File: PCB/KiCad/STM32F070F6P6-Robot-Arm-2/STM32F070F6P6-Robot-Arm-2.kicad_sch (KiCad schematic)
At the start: 37 parts, among them J10 Barrel_Jack_Switch, J6 Conn_01x03_Pin, J7 Conn_01x03_Pin, J8 Conn_01x03_Pin, J9 Conn_01x03_Pin, T14C1_LED1 LED, T1C2_LED1 LED, T1C3_LED1 LED, T3C1_LED1 LED, T3C2_LED1 LED, T3C4_LED1 LED, U1 STM32F070F6Px, U2_AMS1117-3.3 AMS1117-3.3, Y1 8MHz

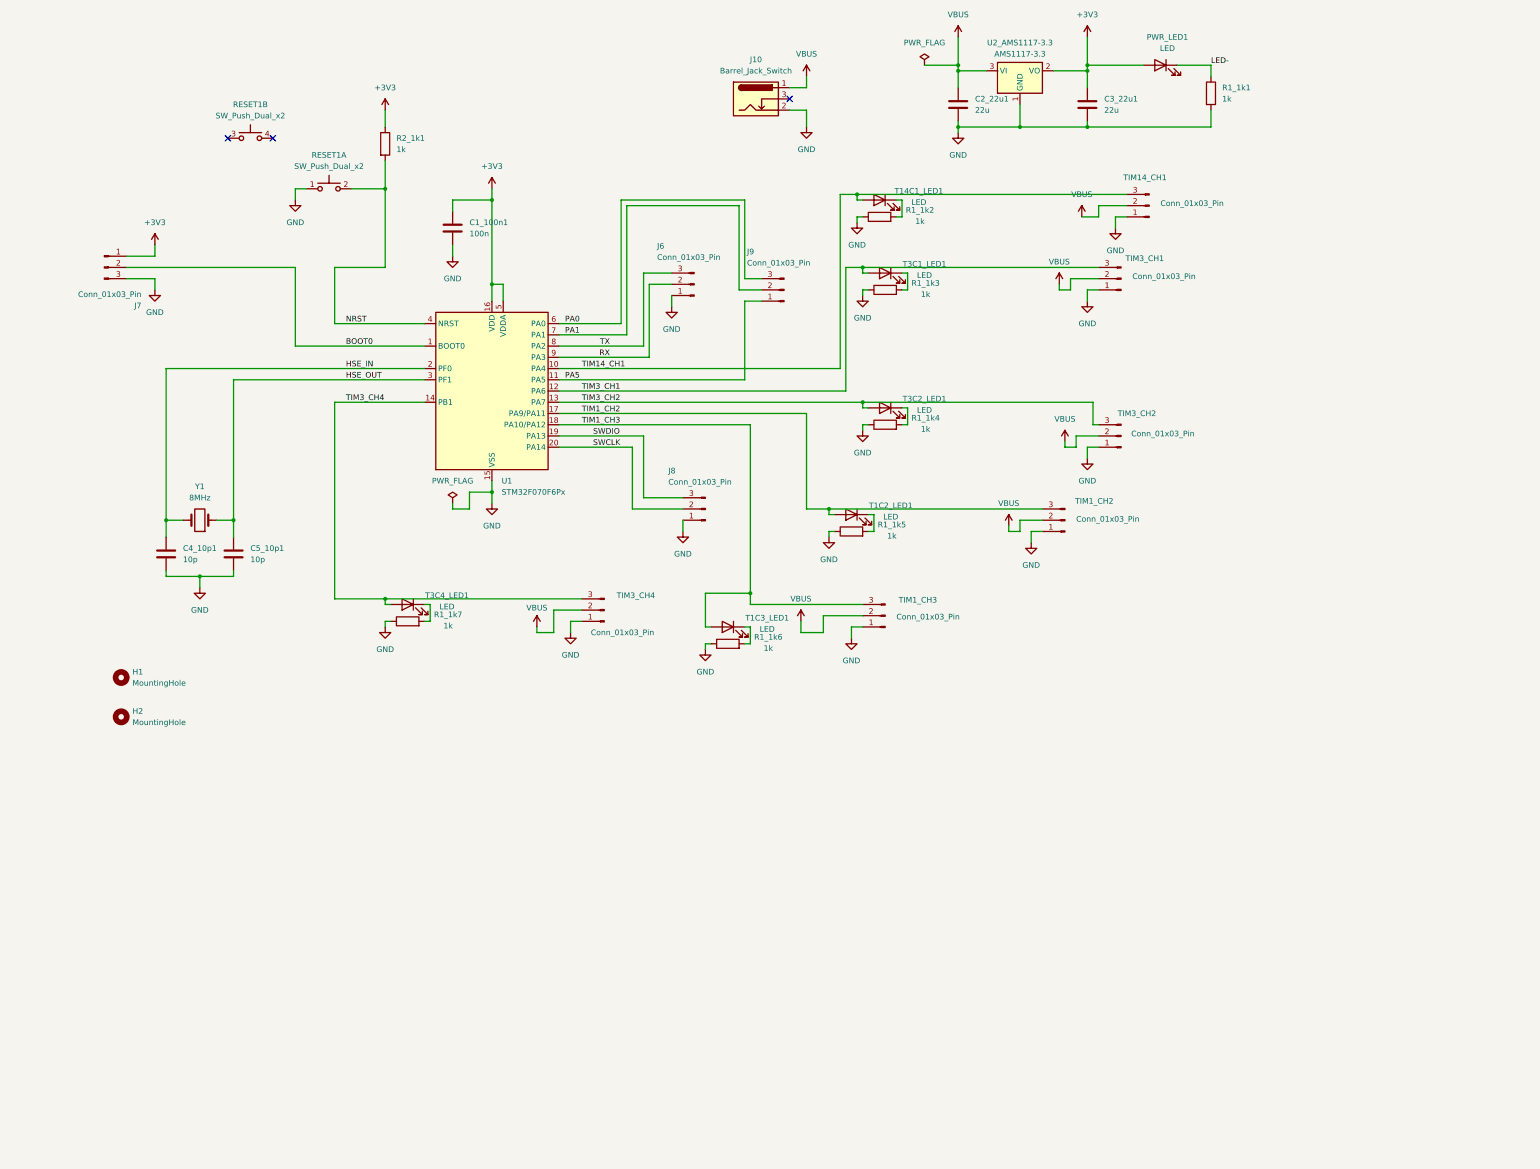
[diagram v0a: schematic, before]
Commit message: Updated schematic
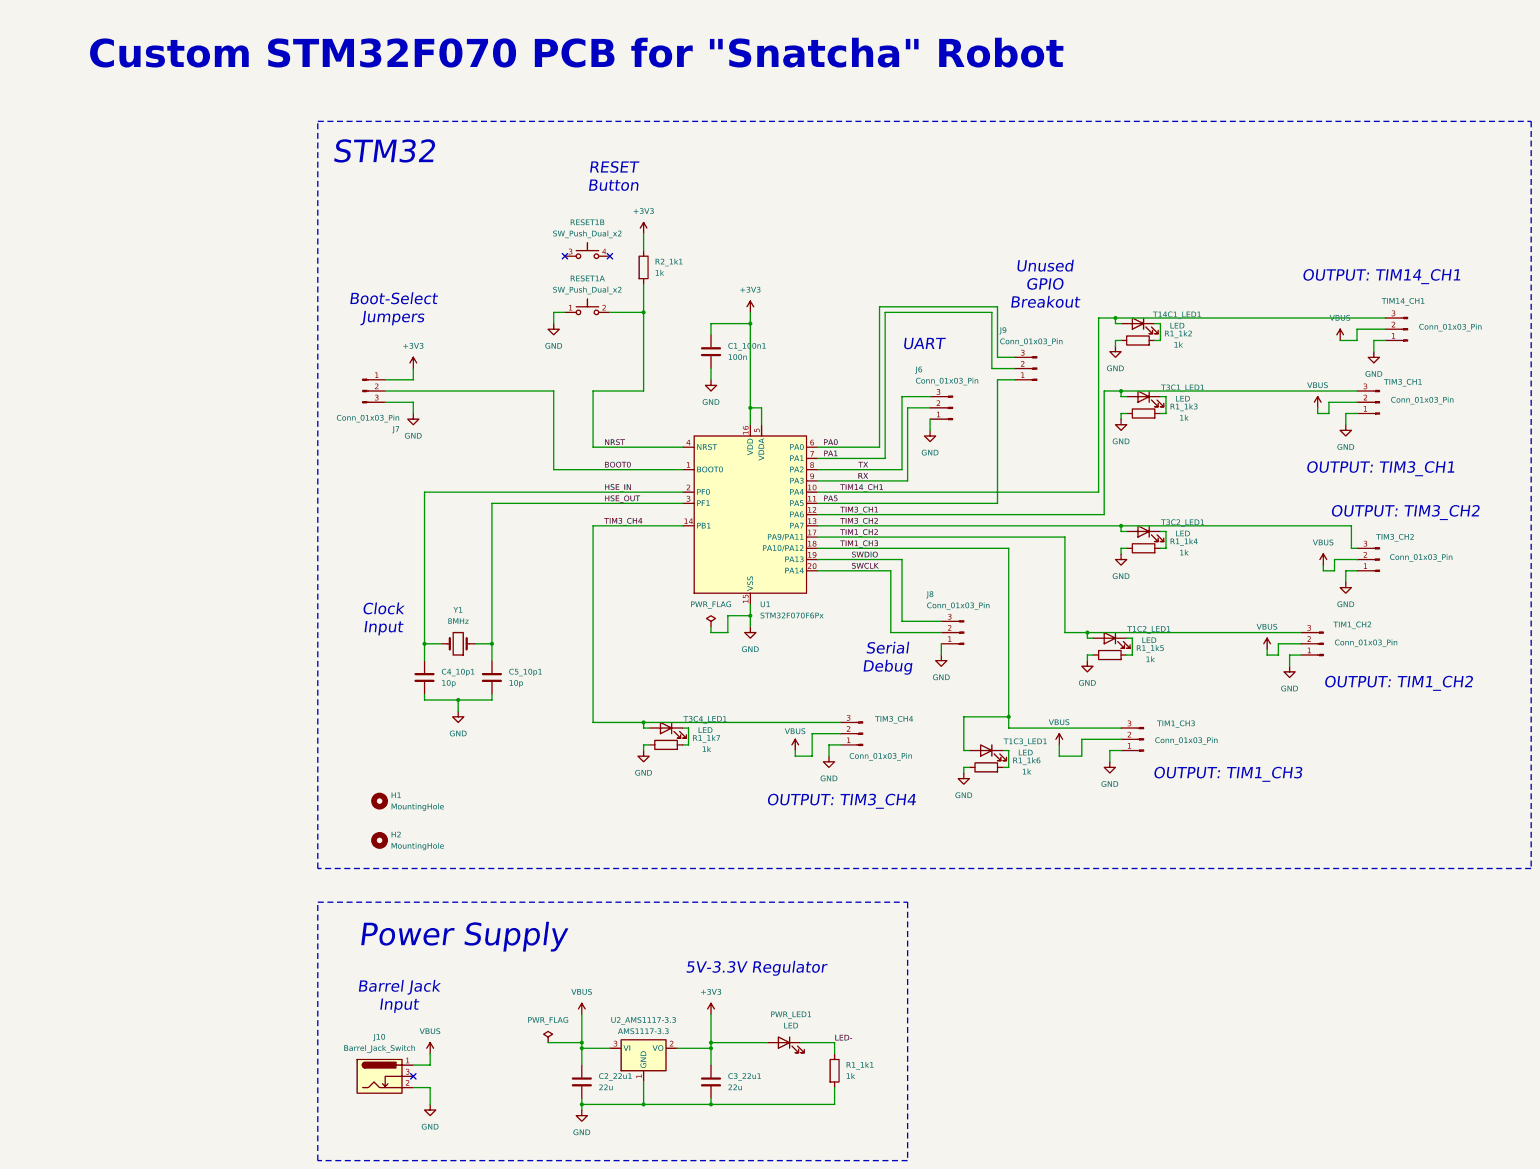
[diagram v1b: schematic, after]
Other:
- note added: "5V-3.3V Regulator"
- note added: "Barrel Jack Input"
- note added: "Boot-Select Jumpers"
- note added: "Clock Input"
- note added: "Custom STM32F070 PCB for "Snatcha" Robot"
- note added: "OUTPUT: TIM14_CH1"
- note added: "OUTPUT: TIM1_CH2"
- note added: "OUTPUT: TIM1_CH3"
- note added: "OUTPUT: TIM3_CH1"
- note added: "OUTPUT: TIM3_CH2"
- note added: "OUTPUT: TIM3_CH4"
- note added: "Power Supply"
- note added: "RESET Button"
- note added: "STM32"
- note added: "Serial Debug"
- note added: "UART"
- note added: "Unused GPIO Breakout"
- company: (none) -> Lachlan Richards
- title: STM32F070F6Px Breakout -> Custom STM32F070 PCB for "Snatcha" Robot
- moved on the sheet: C1_100n1, C2_22u1, C3_22u1, C4_10p1, C5_10p1, H1, H2, J10, J6, J7, J8, J9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
